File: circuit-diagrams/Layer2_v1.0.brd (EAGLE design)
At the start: 38.1 x 50.8 mm, 5 parts

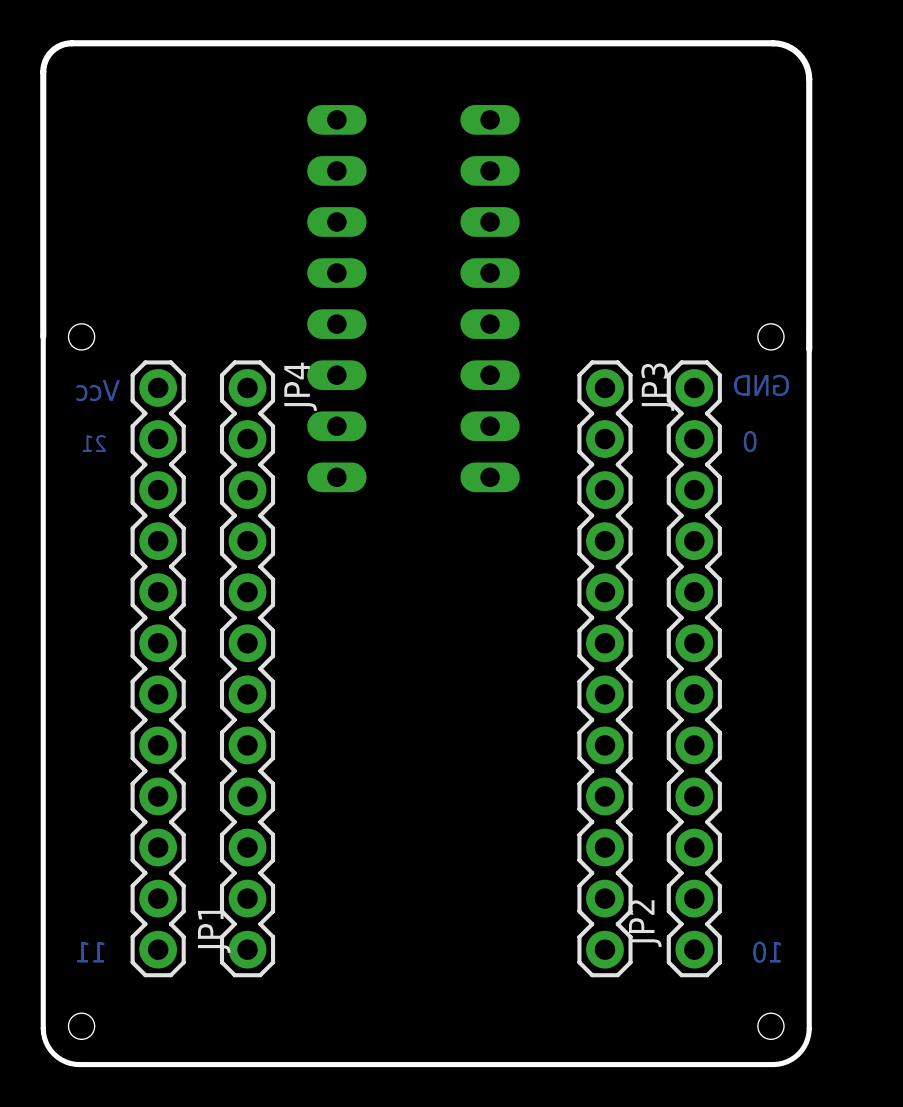
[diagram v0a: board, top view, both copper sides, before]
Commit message: Added Layer2 CircuitCam, Eagle, BoardMaster files
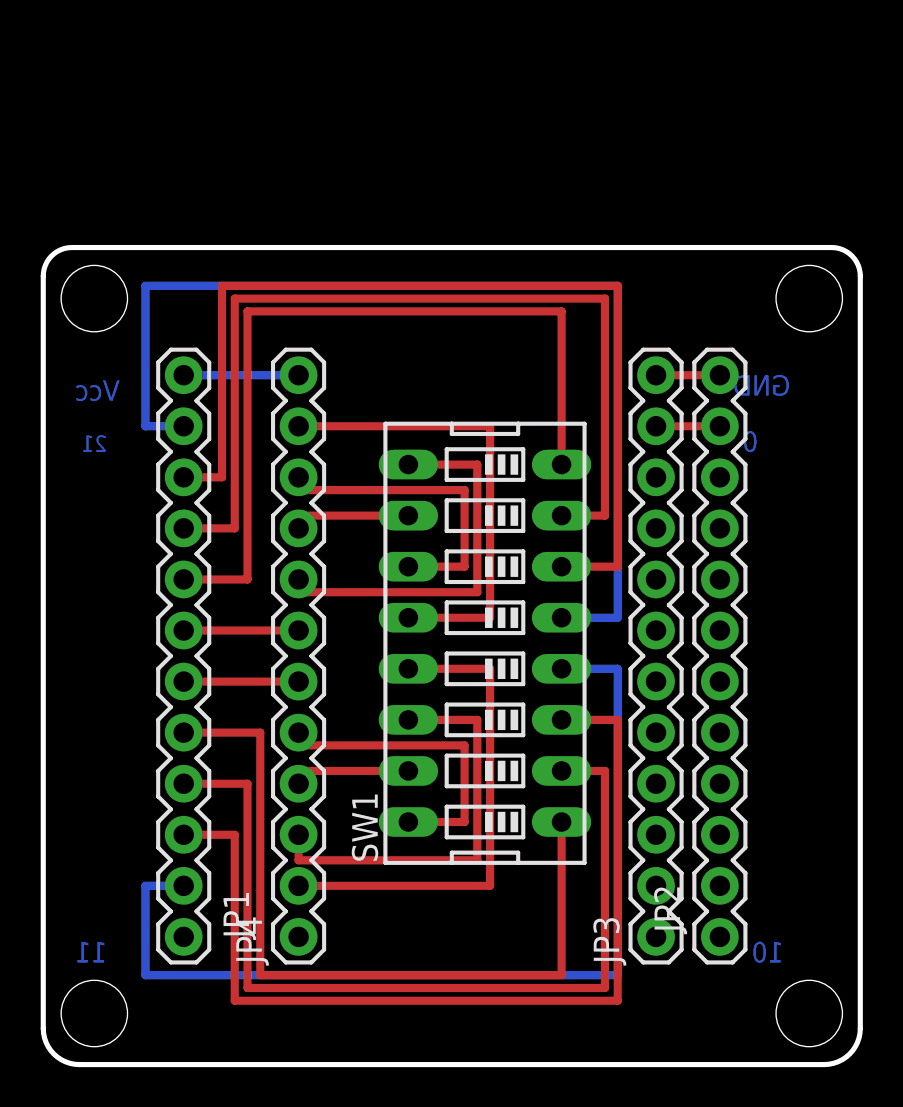
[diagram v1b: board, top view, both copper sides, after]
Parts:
- added JP5, JP6, JP7, JP8: STAND-OFF, SparkFun-Electromechanical:STAND-OFF
- moved JP3 27.4 mm to (30.5, 6.35), turned to 90 degrees
- moved JP4 27.4 mm to (12.7, 6.35), turned to 90 degrees
- moved SW1 17.5 mm to (22.0, 21.0), flipped to the top
- moved JP2 1.42 mm to (33.7, 6.35)
- moved JP1 1.42 mm to (6.99, 6.35)
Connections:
- removed net P0LG: JP2.11
- removed net P10B3: JP2.1, SW1.4
- removed net P11B4: JP1.1, SW1.5
- removed net P12B5: JP1.2, SW1.6
- removed net P19B9: JP1.9
- removed net P1LR: JP2.10
- removed net P20B6: JP1.10, SW1.7
- removed net P21B7: JP1.11, SW1.8
- removed net P2B0: JP2.9, SW1.1
- removed net P3B1: JP2.8, SW1.2
- removed net P4B8: JP2.7
- removed net P9B2: JP2.2, SW1.3
- removed net T10B3: JP3.1, SW1.13
- removed net T11B4: JP4.1, SW1.12
- removed net T12B5: JP4.2, SW1.11
- removed net T20B6: JP4.10, SW1.10
- removed net T21B7: JP4.11, SW1.9
- removed net T2B0: JP3.9, SW1.16
- removed net T3B1: JP3.8, SW1.15
- removed net T9B2: JP3.2, SW1.14
- new net P0LWH: JP2.11, JP3.11
- new net P12B3: JP1.2, SW1.4
- new net P13B2: JP1.3, SW1.3
- new net P14B1: JP1.4, SW1.2
- new net P15B0: JP1.5, SW1.1
- new net P16B8: JP1.6, JP4.6
- new net P17B9: JP1.7, JP4.7
- new net P18B7: JP1.8, SW1.8
- new net P19B6: JP1.9, SW1.7
- new net P20B5: JP1.10, SW1.6
- new net P21B4: JP1.11, SW1.5
- new net T12B3: JP4.2, SW1.13
- new net T13B2: JP4.3, SW1.14
- new net T14B1: JP4.4, SW1.15
- new net T15B0: JP4.5, SW1.16
- new net T18B7: JP4.8, SW1.9
- new net T19B6: JP4.9, SW1.10
- new net T20B5: JP4.10, SW1.11
- new net T21B4: JP4.11, SW1.12
- new net VCC: JP1.12, JP4.12
- net GND: now also JP3.12
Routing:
- net P21B4: track 0.00 -> 51.7 mm
- net P20B5: track 0.00 -> 47.9 mm
- net P12B3: track 0.00 -> 47.9 mm
- net P13B2: track 0.00 -> 46.6 mm
- net P19B6: track 0.00 -> 45.3 mm
- net P14B1: track 0.00 -> 44.1 mm
- net P18B7: track 0.00 -> 39.8 mm
- net P15B0: track 0.00 -> 38.5 mm
- net T12B3: track 0.00 -> 24.4 mm
- net T21B4: track 0.00 -> 23.1 mm
- net T13B2: track 0.00 -> 20.6 mm
- net T18B7: track 0.00 -> 19.3 mm
- net T15B0: track 0.00 -> 15.5 mm
- net T20B5: track 0.00 -> 15.5 mm
- net T14B1: track 0.00 -> 6.10 mm
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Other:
- board size 38.1 x 50.8 mm -> 40.6 x 40.6 mm
